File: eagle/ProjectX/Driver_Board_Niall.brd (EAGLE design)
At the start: 100 x 100 mm, 224 parts, among them IC2 NCV78M05BDTRKG, J1 694102303002, J2 694102303002, U1 TC4427AEOA, U10 TC4427AEOA, U11 TC4427AEOA, U12 TC4427AEOA, U1200 CD74HC4067SM96, U13 TC4427AEOA, U14 TC4427AEOA, U15 TC4427AEOA, U16 TC4427AEOA, U17 TC4427AEOA, U18 TC4427AEOA, U19 TC4427AEOA, U2 TC4427AEOA, U20 TC4427AEOA, U200 ADA4091-2ARZ-RL, U21 TC4427AEOA, U22 TC4427AEOA, U23 TC4427AEOA, U24 TC4427AEOA, U25 TC4427AEOA, U26 TC4427AEOA, U27 TC4427AEOA, U28 TC4427AEOA, U29 TC4427AEOA, U3 TC4427AEOA, U30 TC4427AEOA, U31 TC4427AEOA, U32 TC4427AEOA, U33 TC4427AEOA, U34 TC4427AEOA, U35 TC4427AEOA, U36 TC4427AEOA, U37 TC4427AEOA, U38 TC4427AEOA, U39 TC4427AEOA, U4 TC4427AEOA, U40 TC4427AEOA, U41 TC4427AEOA, U42 TC4427AEOA, U43 TC4427AEOA, U44 TC4427AEOA, U45 TC4427AEOA, U46 TC4427AEOA, U47 TC4427AEOA, U48 TC4427AEOA, U49 TC4427AEOA, U5 TC4427AEOA, U50 TC4427AEOA, U6 TC4427AEOA, U7 TC4427AEOA, U8 TC4427AEOA, U9 TC4427AEOA

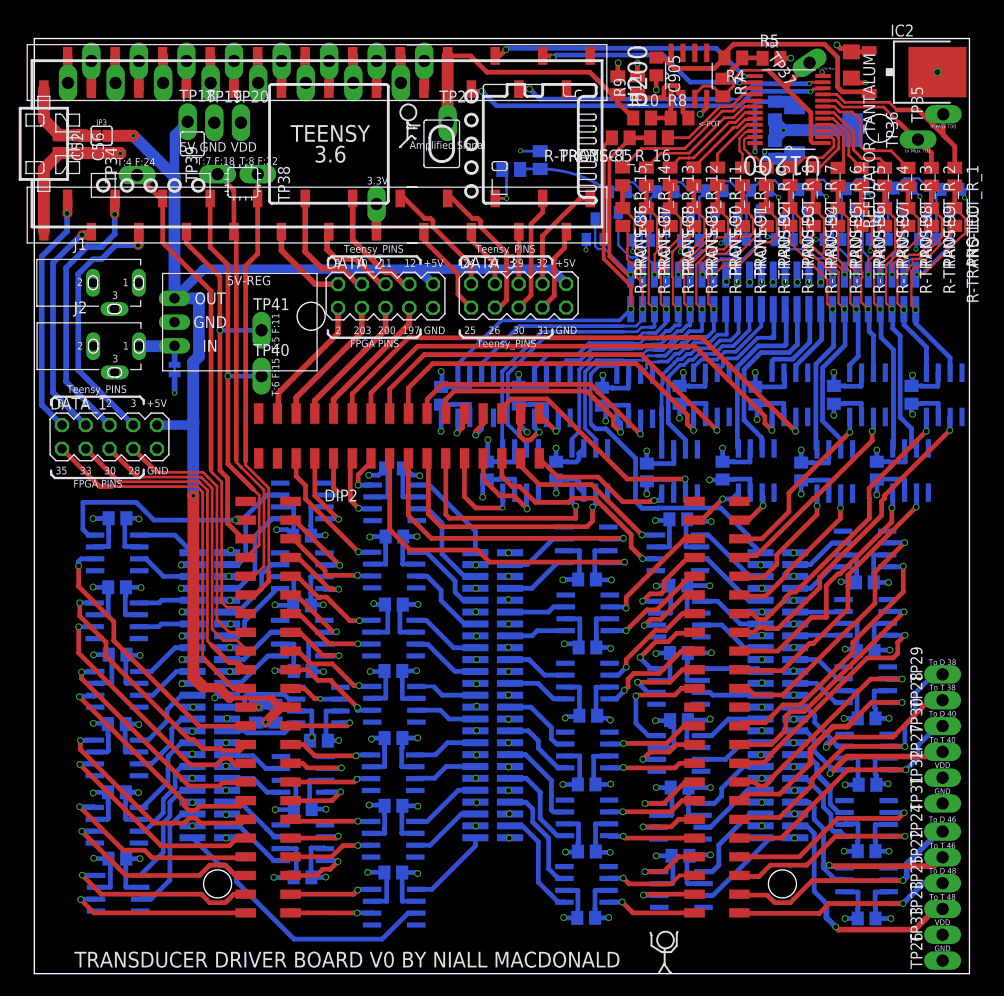
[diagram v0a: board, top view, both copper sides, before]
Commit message: Boards almost done
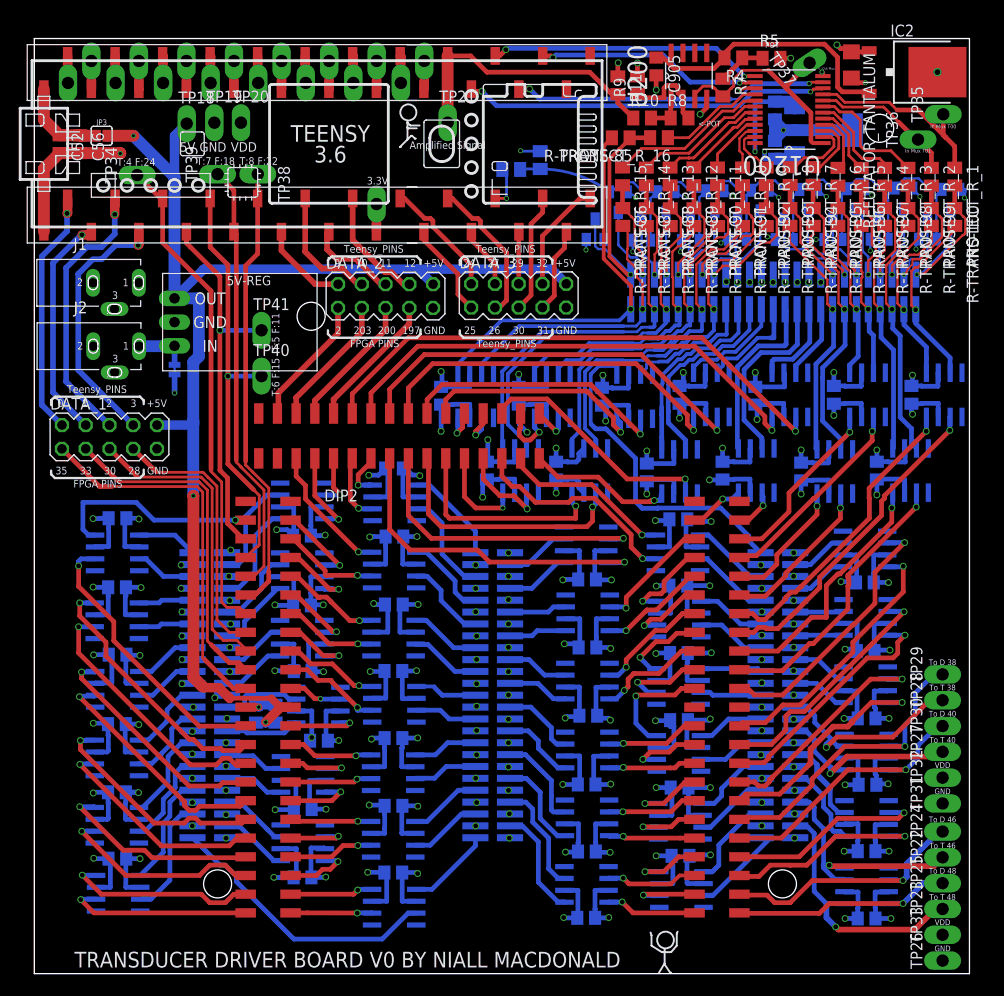
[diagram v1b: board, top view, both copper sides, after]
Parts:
- moved TP18 0.22 mm to (16.3, 90.9)
